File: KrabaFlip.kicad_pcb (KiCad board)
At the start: 2 copper layers, 13 parts, among them J1 522711369, J2 USB4105GFA120, J3 S2B-PH-K-SLFSN, J4 MSD-4-A, U3 CM5108032

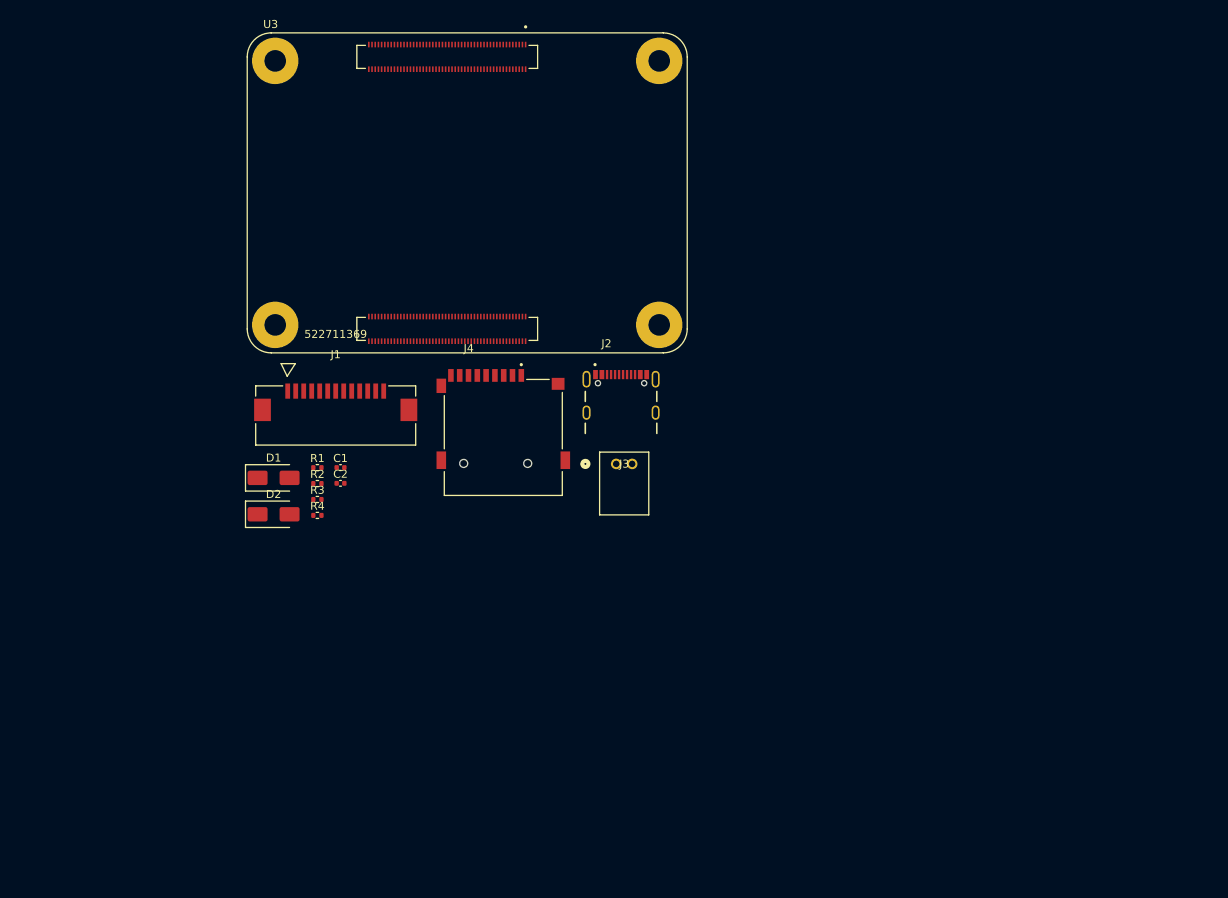
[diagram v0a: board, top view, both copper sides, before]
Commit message: Add KrabaFlip.kicad_pcb
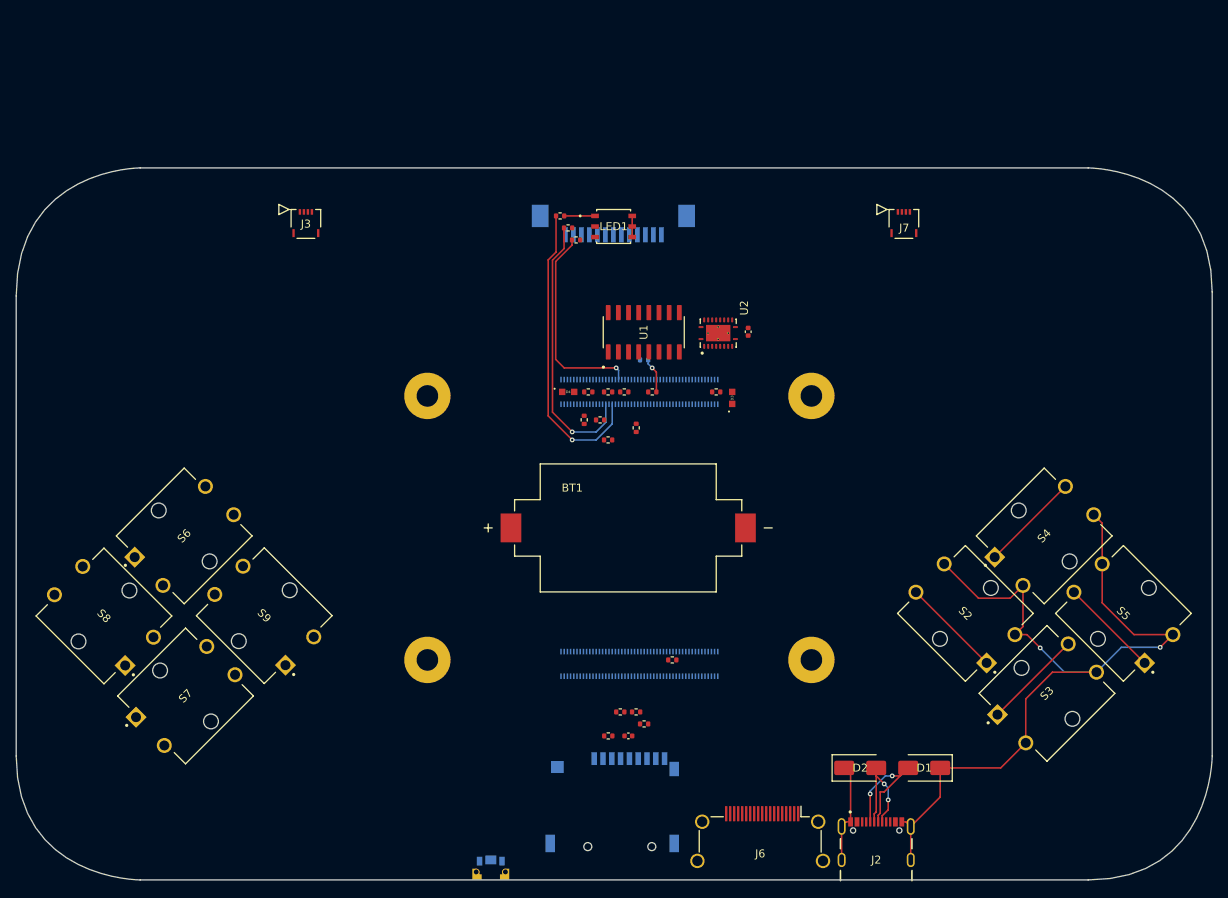
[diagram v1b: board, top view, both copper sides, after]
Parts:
- added BT1: 1060, 1060:BAT_1060, F.Cu at (150.0, 103.5)
- added D3: LTST-C190KFKT, LTST-C190KFKT:LEDM1608X80, F.Cu at (163.0, 87.2)
- added D4: LTST-C190KFKT, LTST-C190KFKT:LEDM1608X80, F.Cu at (142.5, 86.5)
- added J6: HDMI_A, Connector_Video:HDMI_A_Amphenol_10029449-x01xLF_Horizontal, F.Cu at (166.5, 144.2)
- added J7: 5034800440, 5034800440:CON_5034800440_MOL, F.Cu at (184.5, 65.5)
- added LED1: ASMG-PT00-00001, ASMG-PT00-00001:ASMG-PT00_BRA, F.Cu at (148.2, 65.8)
- added R10: 0Ω, Resistor_SMD:R_0402_1005Metric, F.Cu at (144.5, 90.0)
- added R11: 10kΩ, Resistor_SMD:R_0402_1005Metric, F.Cu at (151.0, 91.0)
- added R12: 10kΩ, Resistor_SMD:R_0402_1005Metric, F.Cu at (146.5, 90.0)
- added R13: 10kΩ, Resistor_SMD:R_0402_1005Metric, F.Cu at (147.5, 86.5)
- added R14: 10kΩ, Resistor_SMD:R_0402_1005Metric, F.Cu at (149.5, 86.5)
- added R15: 10kΩ, Resistor_SMD:R_0402_1005Metric, F.Cu at (155.5, 120.0)
- added R16: 10kΩ, Resistor_SMD:R_0402_1005Metric, F.Cu at (147.5, 92.5)
- added R17: 10kΩ, Resistor_SMD:R_0402_1005Metric, F.Cu at (153.0, 86.5)
- added R18: 10kΩ, Resistor_SMD:R_0402_1005Metric, B.Cu at (152.0, 82.5)
- added R5: 1kΩ, Resistor_SMD:R_0402_1005Metric, F.Cu at (141.5, 64.5)
- added R6: 1kΩ, Resistor_SMD:R_0402_1005Metric, F.Cu at (142.5, 66.0)
- added R7: 1kΩ, Resistor_SMD:R_0402_1005Metric, F.Cu at (143.5, 67.5)
- added R8: 1kΩ, Resistor_SMD:R_0402_1005Metric, F.Cu at (145.0, 86.5)
- added R9: 1kΩ, Resistor_SMD:R_0402_1005Metric, F.Cu at (161.0, 86.5)
- added S1: TL6340AF160Q, TL6340AF160Q:SW_TL6340AF160Q, B.Cu at (132.8, 146.5)
- added S2: B3F-4050, B3F_4050:SW_B3F-4050, F.Cu at (192.2, 114.2)
- added S3: B3F-4050, B3F_4050:SW_B3F-4050, F.Cu at (202.3, 124.2)
- added S4: B3F-4050, B3F_4050:SW_B3F-4050, F.Cu at (202.0, 104.5)
- added S5: B3F-4050, B3F_4050:SW_B3F-4050, F.Cu at (211.9, 114.2)
- added S6: B3F-4050, B3F_4050:SW_B3F-4050, F.Cu at (94.5, 104.5)
- added S7: B3F-4050, B3F_4050:SW_B3F-4050, F.Cu at (94.7, 124.5)
- added S8: B3F-4050, B3F_4050:SW_B3F-4050, F.Cu at (84.5, 114.5)
- added S9: B3F-4050, B3F_4050:SW_B3F-4050, F.Cu at (104.5, 114.5)
- added U1: MCP3008-I_SL, MCP3008-I_SL:SOIC127P600X175-16N, F.Cu at (151.9, 79.0)
- added U2: TXS0108ERGYR, TXS0108ERGYR:IC_TXS0108ERGYR, F.Cu at (161.2, 79.2)
- J1, J4, U3: moved to B.Cu
- J3: value S2B-PH-K-SLFSN -> 5034800440; footprint S2B-PH-K-S-LF-SN:CONN_S2B-PH-K-S_JST -> 5034800440:CON_5034800440_MOL
- moved D1 89.0 mm to (187.0, 133.5), turned to 180 degrees
- moved D2 79.9 mm to (179.0, 133.5)
- moved J2 64.4 mm to (181.0, 145.0)
- moved C2 54.4 mm to (165.0, 79.0), turned to 90 degrees
- moved J4 49.8 mm to (148.0, 140.1), turned to 180 degrees
- moved R1 49.5 mm to (147.5, 129.5), turned to 180 degrees
- moved C1 49.2 mm to (150.0, 129.5)
- moved J3 49.0 mm to (109.7, 65.5)
- moved R4 48.5 mm to (152.0, 128.0)
- moved R3 47.9 mm to (151.0, 126.5)
- moved R2 47.4 mm to (149.0, 126.5), turned to 180 degrees
- moved U3 46.0 mm to (148.9, 103.5), turned to 180 degrees
- moved J1 43.2 mm to (148.1, 63.8)
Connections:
- C1 pad 2: USB_DN -> GND
- C2 pad 2: USB_DN -> GND
- D1 pad 1: USB_DN -> GND
- D2 pad 1: USB_DN -> GND
- J1 pad 1: USB_DN -> GND
- J1 pad 10: USB_DN -> GND
- J1 pad 13: USB_DN -> GND
- J1 pad 4: USB_DN -> GND
- J1 pad 7: USB_DN -> GND
- J2 pad A1_B12: USB_DN -> GND
- J2 pad B1_A12: USB_DN -> GND
- J2 pad SH1: USB_DN -> GND
- J2 pad SH2: USB_DN -> GND
- J2 pad SH3: USB_DN -> GND
- J2 pad SH4: USB_DN -> GND
- J3 pad 1: unconnected-(J3-Pad1) -> CPAD1_X
- J3 pad 2: unconnected-(J3-Pad2) -> VBUS
- J4 pad 6: USB_DN -> GND
- J4 pad G1: USB_DN -> GND
- J4 pad G2: USB_DN -> GND
- J4 pad G3: USB_DN -> GND
- J4 pad G4: USB_DN -> GND
- U3 pad 1: USB_DN -> GND
- U3 pad 107: USB_DN -> GND
- U3 pad 108: USB_DN -> GND
- U3 pad 111: unconnected-(U3B-VBUS_EN-Pad111) -> +3V3
- U3 pad 113: USB_DN -> GND
- U3 pad 114: USB_DN -> GND
- U3 pad 119: USB_DN -> GND
- U3 pad 120: USB_DN -> GND
- U3 pad 125: USB_DN -> GND
- U3 pad 126: USB_DN -> GND
- U3 pad 13: USB_DN -> GND
- U3 pad 131: USB_DN -> GND
- U3 pad 132: USB_DN -> GND
- U3 pad 137: USB_DN -> GND
- U3 pad 138: USB_DN -> GND
- U3 pad 14: USB_DN -> GND
- U3 pad 144: USB_DN -> GND
- U3 pad 150: USB_DN -> GND
- U3 pad 151: unconnected-(U3B-HDMI0_CEC-Pad151) -> HDMI_CEC
- U3 pad 153: unconnected-(U3B-HDMI0_HOTPLUG-Pad153) -> HDMI_HPD
- U3 pad 155: USB_DN -> GND
- U3 pad 156: USB_DN -> GND
- U3 pad 161: USB_DN -> GND
- U3 pad 162: USB_DN -> GND
- U3 pad 167: USB_DN -> GND
- U3 pad 168: USB_DN -> GND
- U3 pad 170: unconnected-(U3B-HDMI0_TX2_P-Pad170) -> HDMI_D2P
- U3 pad 172: unconnected-(U3B-HDMI0_TX2_N-Pad172) -> HDMI_D2N
- U3 pad 173: USB_DN -> GND
- U3 pad 174: USB_DN -> GND
- U3 pad 176: unconnected-(U3B-HDMI0_TX1_P-Pad176) -> HDMI_D1P
- U3 pad 178: unconnected-(U3B-HDMI0_TX1_N-Pad178) -> HDMI_D1N
- U3 pad 179: USB_DN -> GND
- U3 pad 180: USB_DN -> GND
- U3 pad 182: unconnected-(U3B-HDMI0_TX0_P-Pad182) -> HDMI_D0P
- U3 pad 184: unconnected-(U3B-HDMI0_TX0_N-Pad184) -> HDMI_D0N
- U3 pad 185: USB_DN -> GND
- U3 pad 186: USB_DN -> GND
- U3 pad 188: unconnected-(U3B-HDMI0_CLK_P-Pad188) -> HDMI_CKP
- U3 pad 190: unconnected-(U3B-HDMI0_CLK_N-Pad190) -> HDMI_CKN
- U3 pad 191: USB_DN -> GND
- U3 pad 192: USB_DN -> GND
- U3 pad 197: USB_DN -> GND
- U3 pad 198: USB_DN -> GND
- U3 pad 199: unconnected-(U3B-HDMI0_SDA-Pad199) -> HDMI_SDA
- U3 pad 2: USB_DN -> GND
- U3 pad 20: unconnected-(U3A-EEPROM_~{WP}-Pad20) -> Net-(U3A-EEPROM_~{WP})
- U3 pad 200: unconnected-(U3B-HDMI0_SCL-Pad200) -> HDMI_SCL
- U3 pad 21: unconnected-(U3A-LED_~{ACTIVITY}-Pad21) -> Net-(U3A-LED_~{ACTIVITY})
- U3 pad 22: USB_DN -> GND
- U3 pad 23: USB_DN -> GND
- U3 pad 24: unconnected-(U3A-GPIO26-Pad24) -> BUTTON_X
- U3 pad 28: unconnected-(U3A-GPIO13-Pad28) -> BUTTON_DWN
- U3 pad 29: unconnected-(U3A-GPIO16-Pad29) -> BUTTON_A
- U3 pad 30: unconnected-(U3A-GPIO6-Pad30) -> LED_G
- U3 pad 31: unconnected-(U3A-GPIO12-Pad31) -> BUTTON_UP
- U3 pad 32: USB_DN -> GND
- U3 pad 33: USB_DN -> GND
- U3 pad 34: unconnected-(U3A-GPIO5-Pad34) -> LED_R
- U3 pad 37: unconnected-(U3A-GPIO7-Pad37) -> LED_B
- U3 pad 41: unconnected-(U3A-GPIO25-Pad41) -> BUTTON_B
- U3 pad 42: USB_DN -> GND
- U3 pad 43: USB_DN -> GND
- U3 pad 45: unconnected-(U3A-GPIO24-Pad45) -> ADC_3V3_MISO
- U3 pad 46: unconnected-(U3A-GPIO22-Pad46) -> ADC_3V3_CLK
- U3 pad 47: unconnected-(U3A-GPIO23-Pad47) -> ADC_3V3_MOSI
- U3 pad 48: unconnected-(U3A-GPIO27-Pad48) -> BUTTON_Y
- U3 pad 51: unconnected-(U3A-GPIO15-Pad51) -> BUTTON_RGT
- U3 pad 52: USB_DN -> GND
- U3 pad 53: USB_DN -> GND
- U3 pad 55: unconnected-(U3A-GPIO14-Pad55) -> BUTTON_LFT
- U3 pad 59: USB_DN -> GND
- U3 pad 60: USB_DN -> GND
- U3 pad 65: USB_DN -> GND
- U3 pad 66: USB_DN -> GND
- U3 pad 7: USB_DN -> GND
- U3 pad 71: USB_DN -> GND
- U3 pad 74: USB_DN -> GND
- U3 pad 76: unconnected-(U3A-VBAT-Pad76) -> +BATT
- U3 pad 78: unconnected-(U3A-GPIO_VREF-Pad78) -> +3V3
- U3 pad 8: USB_DN -> GND
- U3 pad 88: +3V3 -> CM5_1.8V(OUTPUT)
- U3 pad 89: VBUS -> +3V3
- U3 pad 90: +3V3 -> CM5_1.8V(OUTPUT)
- U3 pad 91: VBUS -> +3V3
- U3 pad 92: unconnected-(U3A-PWR_BUTTON-Pad92) -> Net-(U3A-PWR_BUTTON)
- U3 pad 95: unconnected-(U3A-LED_~{PWR}-Pad95) -> Net-(U3A-LED_~{PWR})
- U3 pad 98: USB_DN -> GND
- U3 pad 99: unconnected-(U3A-PMIC_ENABLE-Pad99) -> +3V3
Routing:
- net GND: track 0.00 -> 121.8 mm, vias 0 -> 2
- net LED_R: track 0.00 -> 37.9 mm, vias 0 -> 1
- net LED_G: track 0.00 -> 34.1 mm, vias 0 -> 1
- net LED_B: track 0.00 -> 25.4 mm, vias 0 -> 1
- net USB_DN: track 0.00 -> 18.4 mm, vias 0 -> 2
- net USB_DP: track 0.00 -> 14.5 mm, vias 0 -> 2
- net BUTTON_X: track 0.00 -> 12.5 mm
- net BUTTON_B: track 0.00 -> 12.5 mm
- net BUTTON_Y: track 0.00 -> 12.5 mm
- net BUTTON_A: track 0.00 -> 12.5 mm
- net +3V3: track 0.00 -> 4.42 mm, vias 0 -> 1
- net Net-(LED1-Pad1): track 0.00 -> 3.85 mm
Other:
- board outline added: 149.5 x 89 mm
